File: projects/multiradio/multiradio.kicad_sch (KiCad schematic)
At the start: 23 parts, among them J1 USB_B

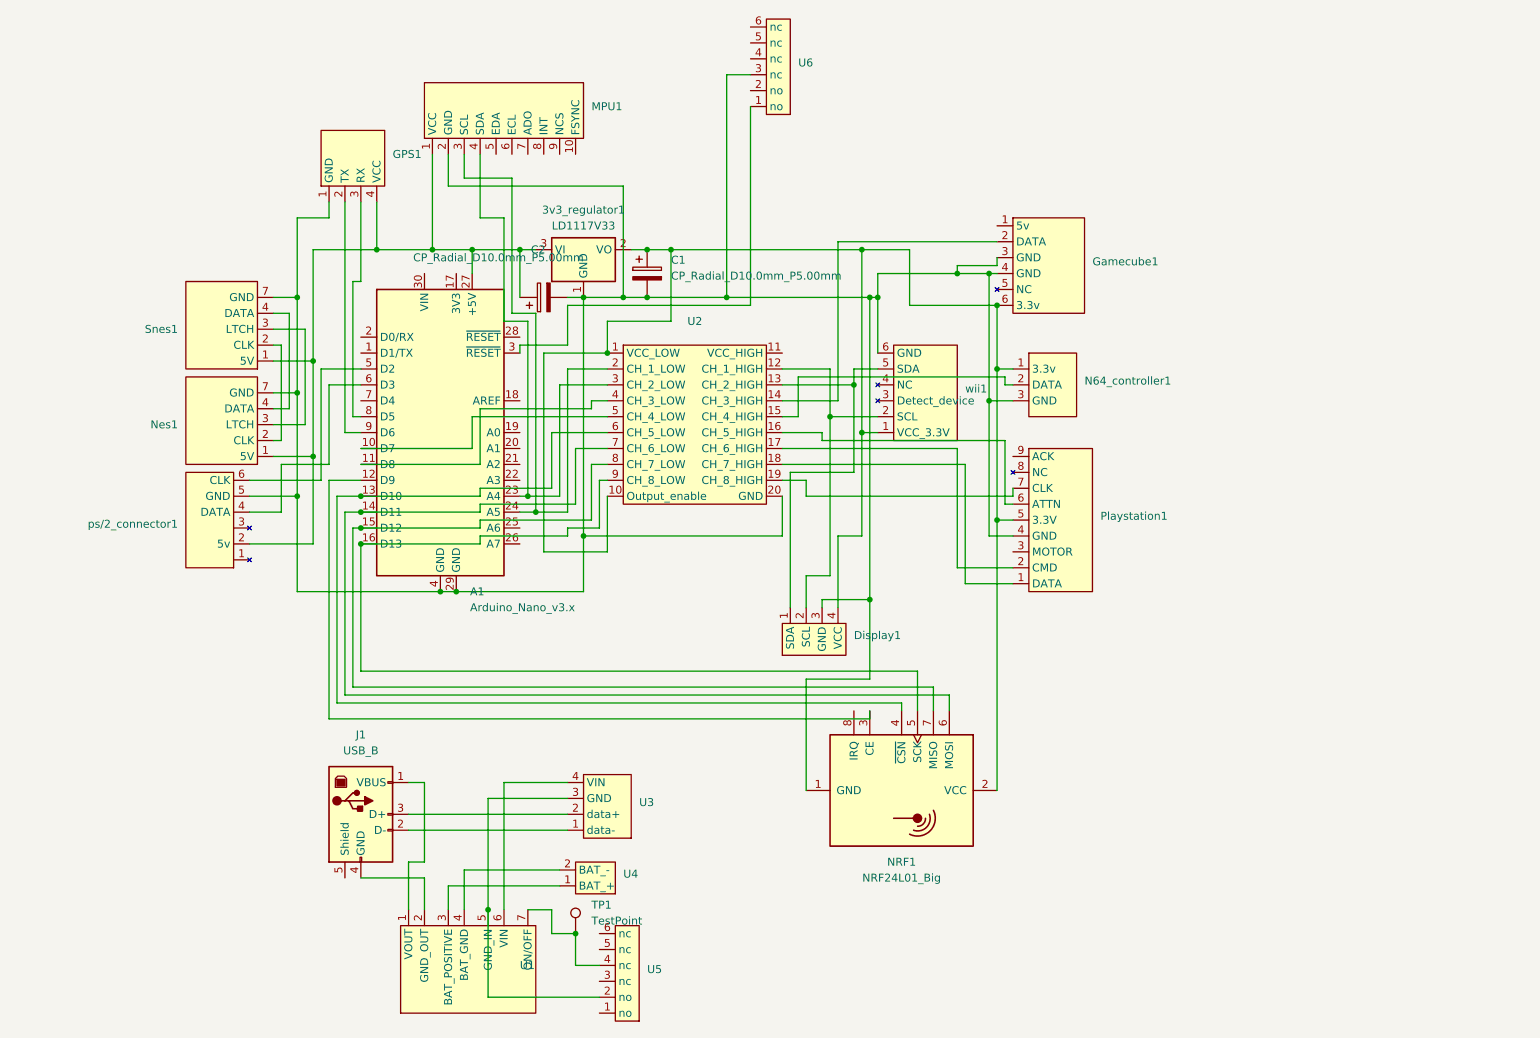
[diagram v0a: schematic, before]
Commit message: only multi remote left
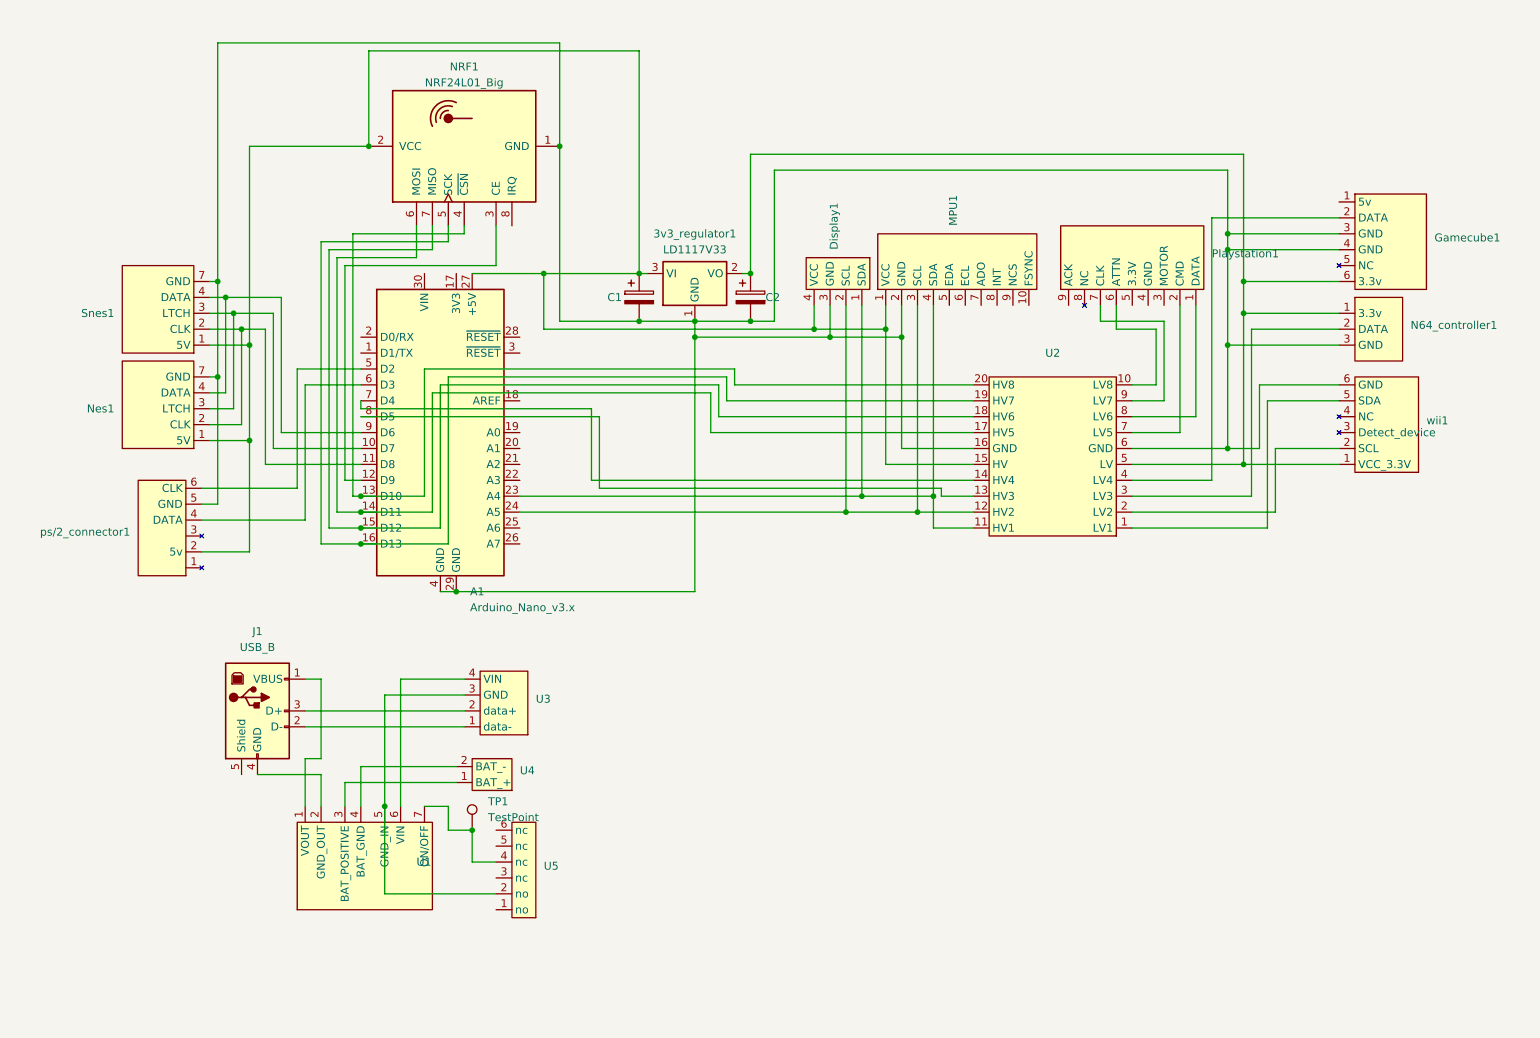
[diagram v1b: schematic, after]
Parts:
- removed GPS1: ~, Footprints_cez:GY-NEO6MV2, symbol Symbols_cez:GY-NEO6MV2
- removed U2: ~, Footprints_cez:TXS0108E, symbol Symbols_cez:TXS0108E_
- removed U6: ~, Footprints_cez:Switch A03 PS-22F03, symbol Symbols_cez:Switch_A03_PS-22F03
- added U2: ~, Footprints_cez:8 Channel Logic Level Converter, symbol Symbols_cez:8_Channel_Logic_Level_Converter
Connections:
- net at Gamecube1.2 (DATA): now also U2.4 (LV4)
- net at 3v3_regulator1.1 (GND), A1.29 (GND), A1.4 (GND)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: now also U2.16 (GND), U2.6 (GND); no longer Playstation1.4 (GND)
- net at 3v3_regulator1.2 (VO), Gamecube1.6 (3.3v), N64_controller1.1 (3.3v)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: now also C2.1, U2.5 (LV); no longer C1.1, Display1.4 (VCC), NRF1.2 (VCC), Playstation1.5 (3.3V)
- net at wii1.2 (SCL): now also U2.2 (LV2); no longer Display1.2 (SCL)
- net at wii1.5 (SDA): now also U2.1 (LV1); no longer Display1.1 (SDA)
- net at 3v3_regulator1.3 (VI), A1.27 (+5V), MPU1.1 (VCC)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: now also C1.1, Display1.4 (VCC), NRF1.2 (VCC), U2.15 (HV); no longer C2.1
- net at A1.24 (A5), MPU1.3 (SCL): now also Display1.2 (SCL), U2.12 (HV2)
- net at A1.23 (A4), MPU1.4 (SDA): now also Display1.1 (SDA), U2.11 (HV1)
- net at A1.10 (D7): now also Nes1.3 (LTCH), Snes1.3 (LTCH)
- net at A1.11 (D8): now also Nes1.2 (CLK), Snes1.2 (CLK)
- net at A1.13 (D10), NRF1.4 (~{CSN}): now also U2.20 (HV8)
- net at A1.14 (D11), NRF1.6 (MOSI): now also U2.17 (HV5)
- net at A1.15 (D12), NRF1.7 (MISO): now also U2.18 (HV6)
- net at A1.16 (D13), NRF1.5 (SCK): now also U2.19 (HV7)
- net at A1.7 (D4): now also U2.14 (HV4)
- net at A1.8 (D5): now also U2.13 (HV3)
- net at A1.9 (D6): now also Nes1.4 (DATA), Snes1.4 (DATA)
- net at N64_controller1.2 (DATA): now also U2.3 (LV3)
- net at Playstation1.6 (ATTN): now also U2.10 (LV8)
- net at Playstation1.2 (CMD): now also U2.7 (LV5)
- net at Playstation1.1 (DATA): now also U2.8 (LV6)
- net at Playstation1.7 (CLK): now also U2.9 (LV7)
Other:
- moved on the sheet: 3v3_regulator1, C1, C2, Display1, Gamecube1, J1, MPU1, N64_controller1, NRF1, Nes1, Playstation1, Snes1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

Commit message: ps2 180 degree
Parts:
- Playstation1: footprint Footprints_cez:Playstation 2 controller 90 degree -> Footprints_cez:Playstation 2 controller 180
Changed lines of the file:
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@@
 			)
 		)
-		(property "Footprint" "Footprints_cez:Playstation 2 controller 90 degree"
+		(property "Footprint" "Footprints_cez:Playstation 2 controller 180"
 			(at 194.564 25.654 0)
 			(effects
